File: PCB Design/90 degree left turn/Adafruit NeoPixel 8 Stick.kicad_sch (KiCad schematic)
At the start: 7 parts, among them CN1 1X4SMT, CN2 1X4SMT

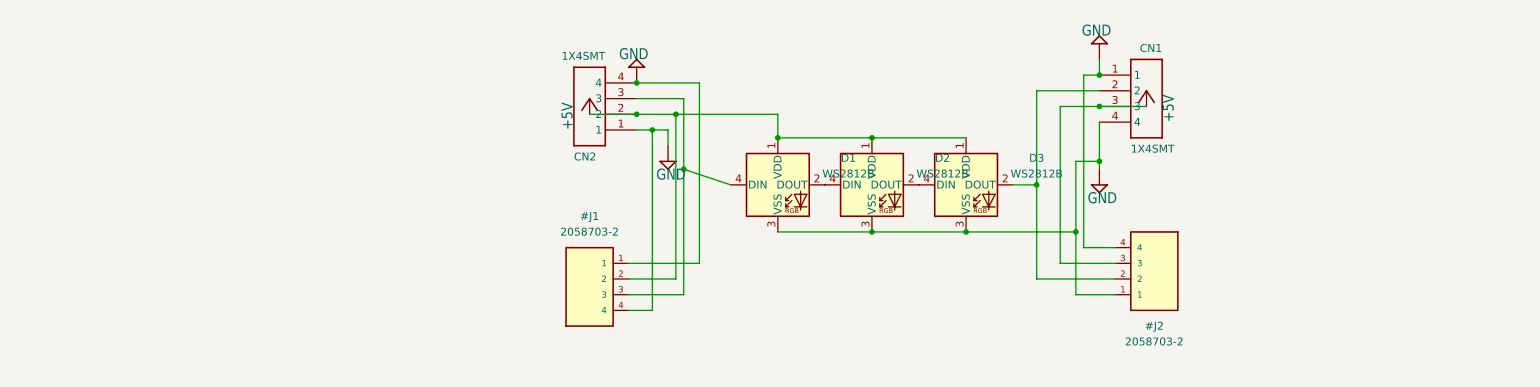
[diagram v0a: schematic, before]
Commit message: 6 pin
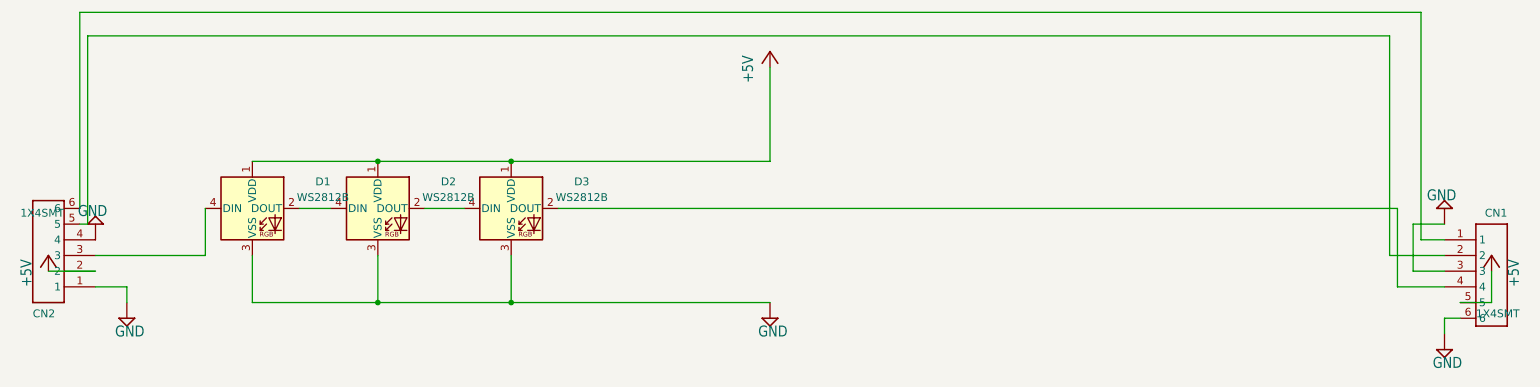
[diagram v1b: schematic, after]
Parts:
- removed #J1, #J2: 2058703-2, TE_2058703-2, symbol 2058703-2:2058703-2
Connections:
- net +5V: now also CN1.5; no longer CN1.3
- net GND: now also CN1.3, CN1.6; no longer CN1.1, CN1.4
- net at D3.2 (DOUT): now also CN1.4; no longer CN1.2
- new net: CN1.2, CN2.5
- new net: CN1.1, CN2.6
